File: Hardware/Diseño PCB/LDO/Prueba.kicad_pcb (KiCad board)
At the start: 2 copper layers, 98.5 x 100.5 mm, 60 parts, among them Q1 2N3904, Q10 BC557, Q11 BC547, Q12 BC557, Q13 BC557, Q14 BC547, Q15 BC557, Q16 BC547, Q17 BC557, Q18 BC547, Q19 BC547, Q2 BC547, Q3 BC547, Q4 BC557, Q5 BC557, Q6 BC547, Q7 BC547, Q8 IRF4905, Q9 BC547, U1 TL431LP, U4 LM324

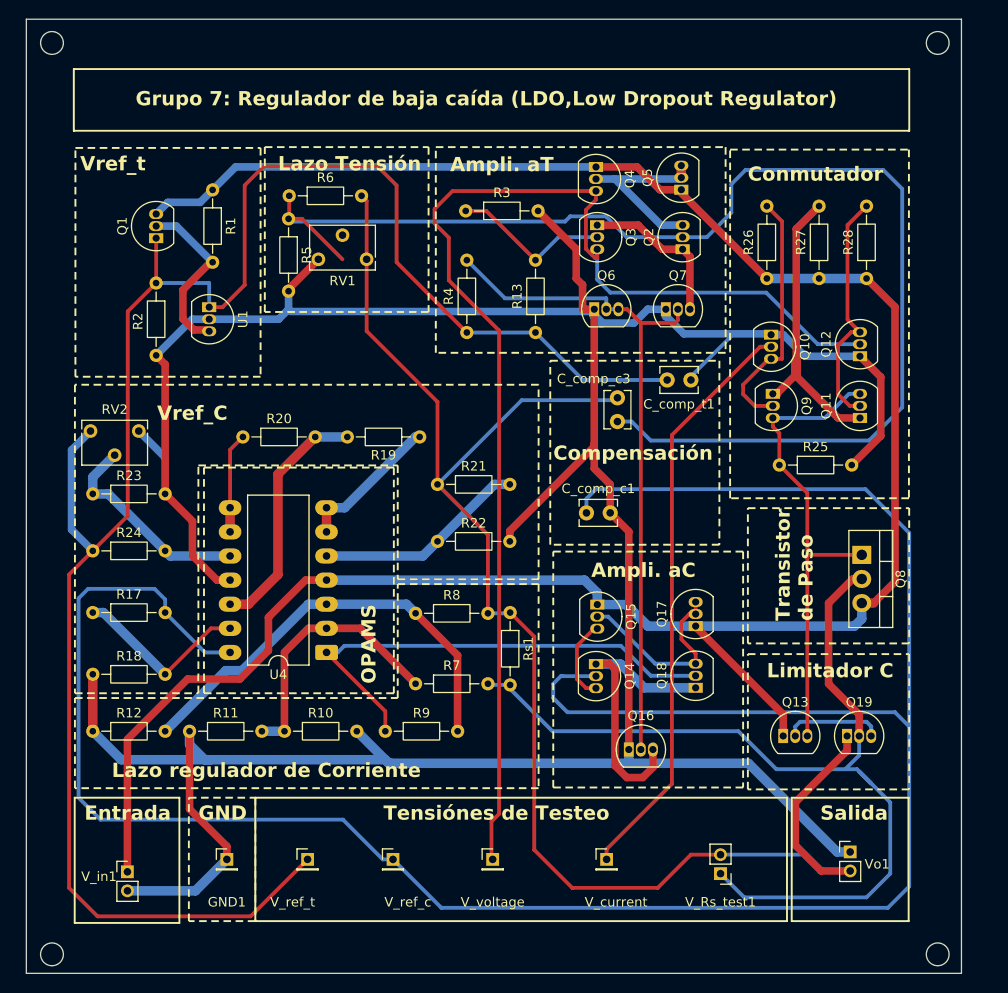
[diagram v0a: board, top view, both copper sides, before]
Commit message: Informe y borneras
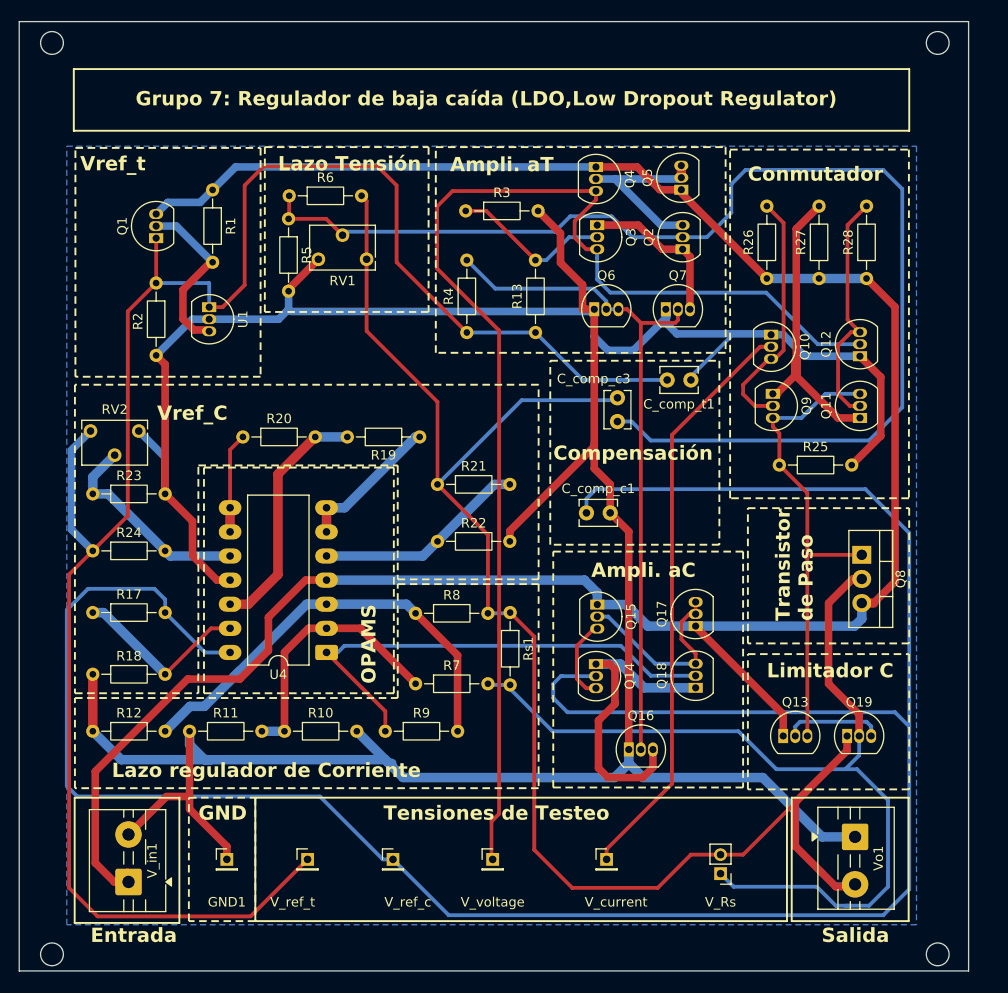
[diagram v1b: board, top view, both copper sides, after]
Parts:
- V_in1, Vo1: footprint Connector_PinHeader_2.00mm:PinHeader_1x02_P2.00mm_Vertical -> TerminalBlock:TerminalBlock_MaiXu_MX126-5.0-02P_1x02_P5.00mm
- moved Vo1 1.67 mm to (141.5, 223.2), turned to -90 degrees
- moved V_in1 1.08 mm to (65.0, 228.0), turned to 90 degrees
- renumbered V_Rs_test1 to V_Rs
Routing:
- net Vcc: track 239.6 -> 245.5 mm
- net VF_fv: track 136.6 -> 130.7 mm
- net GND: track 347.0 -> 349.7 mm
- net -V_Rs: track 159.0 -> 161.6 mm
- net Net-(Q14-E): track 30.8 -> 33.4 mm
- net +V_Rs: track 102.9 -> 101.0 mm
- net Vref_c: track 254.3 -> 256.2 mm
- net Net-(U4A-+): track 46.6 -> 47.6 mm
- net V_voltage: track 132.2 -> 131.7 mm
- added copper zone on B.Cu, net GND
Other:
- board size 98.5 x 100.5 mm -> 100 x 100 mm
- board text added: "Tensiones de Testeo"
- board text removed: "Tensiónes de Testeo"
